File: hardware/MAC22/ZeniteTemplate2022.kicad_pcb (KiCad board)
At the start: 2 copper layers, 130.2 x 52.1 mm, 51 parts, among them J401 USART, J601 RJ45, J602 RJ45, U201 MCP2551-I/SN, U202 MCP2515-xSO, U401 ATMEGA328P-PU, U501 LM7805, Y201 16MHz, Y401 16MHz

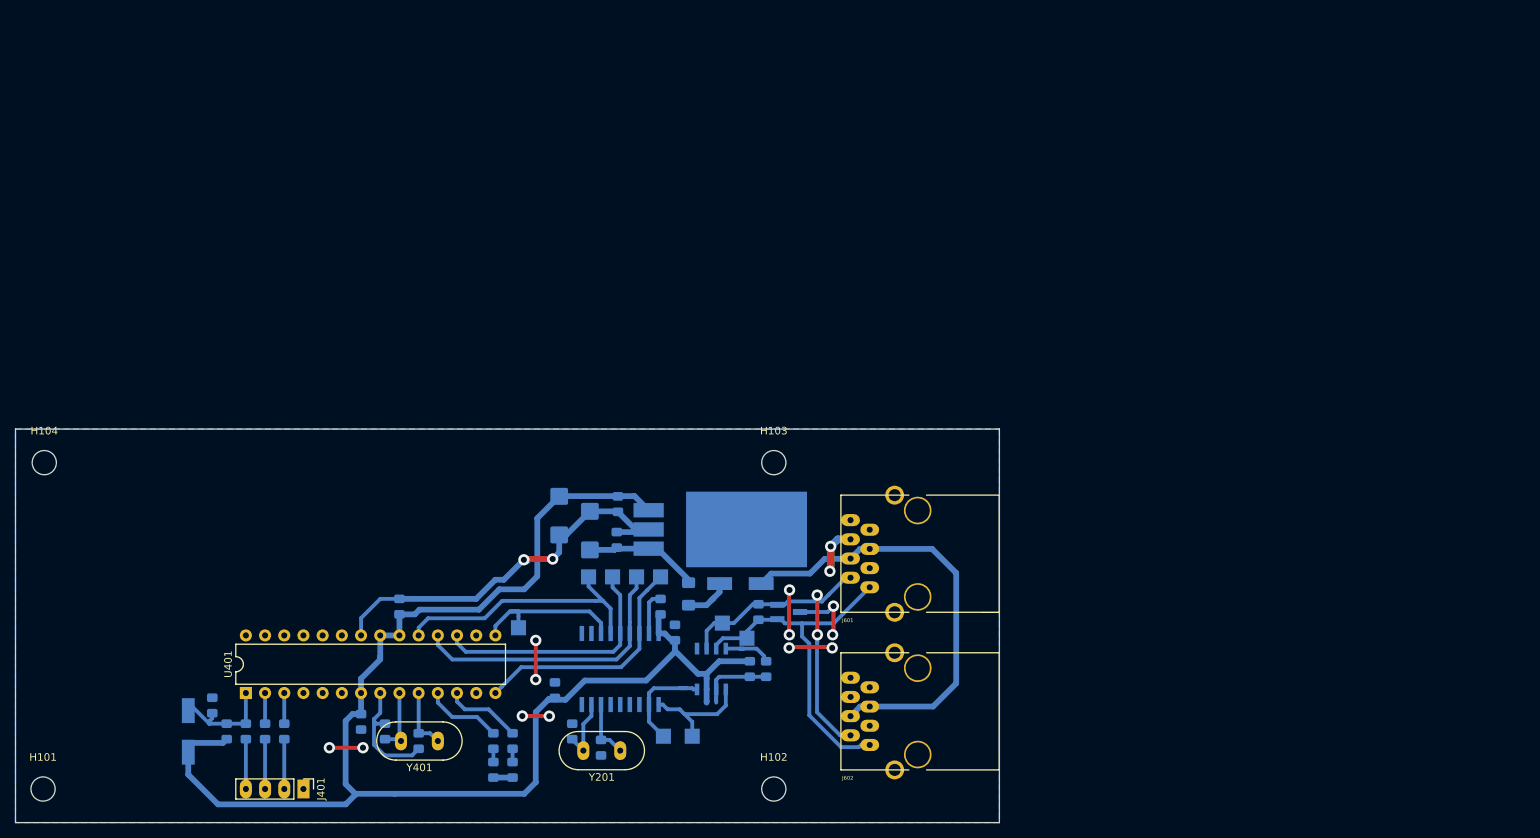
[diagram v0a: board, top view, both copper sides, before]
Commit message: final version PCB
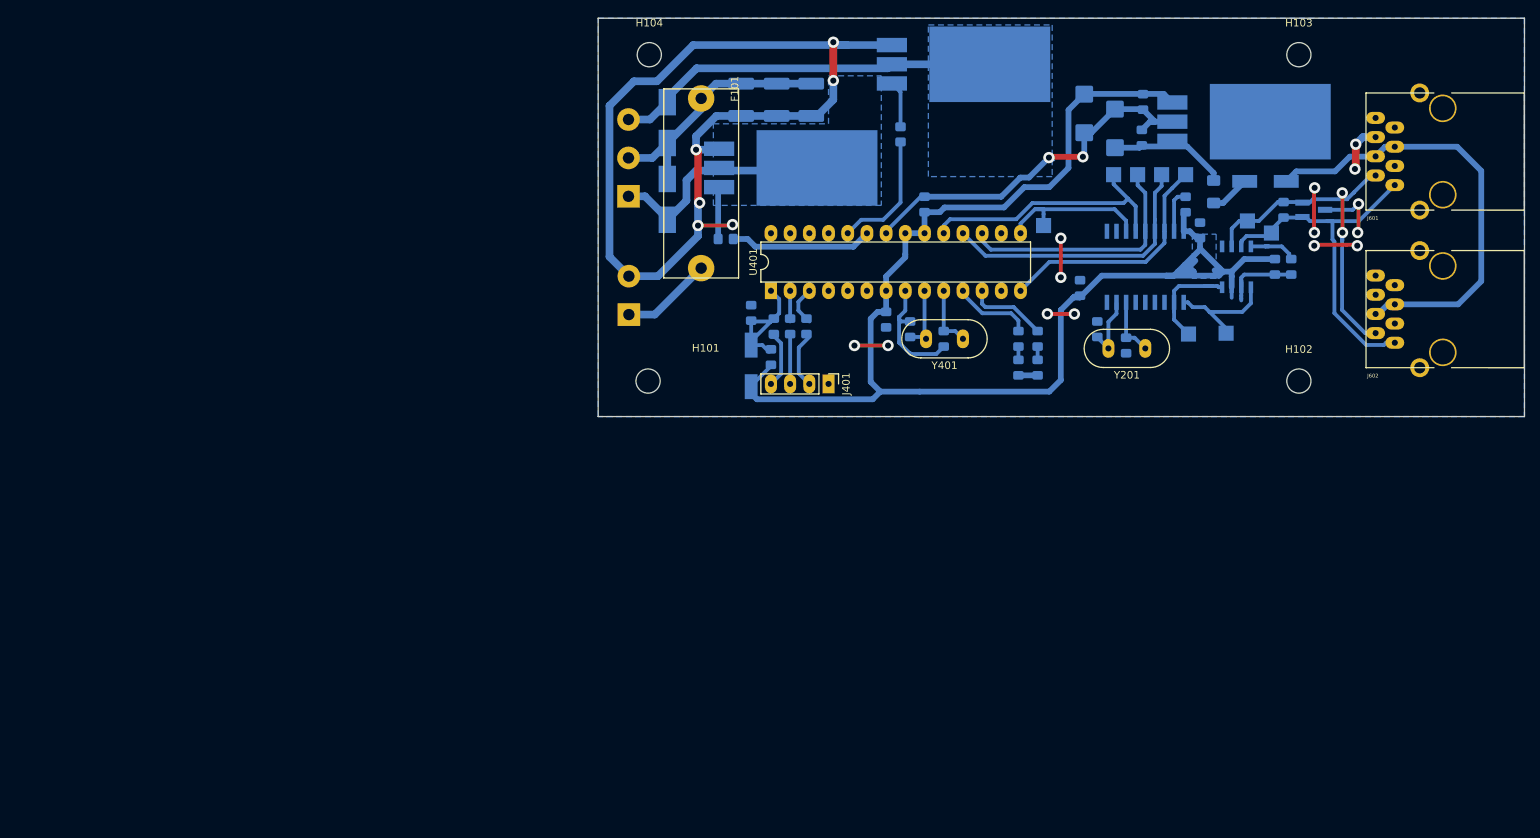
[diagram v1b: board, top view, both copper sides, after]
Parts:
- added C101: 4.7uF, Capacitor_SMD:C_1812_4532Metric_Pad1.57x3.40mm_HandSolder, B.Cu at (180.5, 29.2)
- added C102: 4.7uF, Capacitor_SMD:C_1812_4532Metric_Pad1.57x3.40mm_HandSolder, B.Cu at (185.0, 29.2)
- added C103: 4.7uF, Capacitor_SMD:C_1812_4532Metric_Pad1.57x3.40mm_HandSolder, B.Cu at (175.8, 29.2)
- added D202: 3A, Diode_SMD:D_SMB_Handsoldering, B.Cu at (166.0, 42.4)
- added D502: 3A, Diode_SMD:D_SMB_Handsoldering, B.Cu at (166.0, 32.2)
- added F101: 3A, KicadZeniteSolarLibrary18:Fuse_Holder_5x20, F.Cu at (175.4, 27.8)
- added J101: Conn_01x03, TerminalBlock:TerminalBlock_bornier-3_P5.08mm, B.Cu at (160.9, 42.0)
- added J102: +12V, TerminalBlock:TerminalBlock_bornier-2_P5.08mm, B.Cu at (160.9, 57.6)
- added Q201: IRF530, KicadZeniteSolarLibrary18:TO-220-3_Horizontal_TabDown_SMD, B.Cu at (174.1, 40.8)
- added Q501: IRF530, KicadZeniteSolarLibrary18:TO-220-3_Horizontal_TabDown_SMD, B.Cu at (197.0, 27.1)
- added R204: 100, Resistor_SMD:R_0805_2012Metric_Pad1.20x1.40mm_HandSolder, B.Cu at (173.7, 47.6)
- added R501: 100, Resistor_SMD:R_0805_2012Metric_Pad1.20x1.40mm_HandSolder, B.Cu at (196.8, 33.8)
- moved H101 96.5 mm to (163.4, 66.4)
- moved H104 96.5 mm to (163.6, 23.2)
- moved D401 88.8 mm to (177.1, 64.4)
- moved TP203 88.5 mm to (239.9, 60.1)
- moved C406 88.2 mm to (177.1, 57.4)
- moved C405 88.0 mm to (180.1, 59.2)
- moved H102 88.0 mm to (249.6, 66.4)
- moved H103 88.0 mm to (249.6, 23.2)
- moved U501 87.8 mm to (234.1, 34.6)
- moved R402 87.7 mm to (182.2, 59.2)
- moved J401 87.7 mm to (187.3, 66.8)
- moved TP207 87.7 mm to (245.9, 46.8)
- moved C502 87.5 mm to (228.8, 34.2)
- moved C503 87.5 mm to (228.9, 29.5)
- moved C504 87.5 mm to (221.2, 31.0)
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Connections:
- U401 pad 23: /MCU/analog1 -> /MCU/ONCoil1
- U401 pad 24: unconnected-(U401-Pad24) -> /MCU/ONCoil2
- U501 pad : (no net) -> GND
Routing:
- net GND: track 123.9 -> 249.8 mm, vias 16 -> 22
- net /coil1_drive/Coil-: track 0.00 -> 51.2 mm
- net +12V: track 0.00 -> 35.2 mm
- net /coil2_drive/Coil-: track 0.00 -> 31.3 mm
- net /MCU/ONCoil1: track 0.00 -> 19.7 mm
- net /MCU/ONCoil2: track 0.00 -> 16.7 mm
- net Net-(J102-Pad1): track 0.00 -> 12.4 mm
- net Net-(Q201-Pad1): track 0.00 -> 6.91 mm
- net Net-(Q501-Pad1): track 0.00 -> 6.71 mm
- net /MCU/RESET: track 14.2 -> 18.5 mm
- net +5V: track 186.4 -> 189.1 mm
- net Net-(C405-Pad2): track 6.59 -> 8.01 mm
- net /MCU/USART_TX: track 4.06 -> 5.25 mm
- net Net-(J401-Pad2): track 6.59 -> 7.75 mm
- net Net-(D501-Pad1): track 6.35 -> 5.29 mm
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- added copper zone on B.Cu, net +5V
- added copper zone on B.Cu, net /coil1_drive/Coil-
- added copper zone on B.Cu, net /coil2_drive/Coil-
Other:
- board size 130.2 x 52.1 mm -> 122.6 x 52.7 mm
